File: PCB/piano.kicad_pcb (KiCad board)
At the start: 2 copper layers, 100 x 90 mm, 35 parts, among them J1 Conn_01x02, J2 Conn_01x04, J3 Conn_01x04, SW1 0, SW10 9, SW11 A, SW12 B, SW13 C, SW14 D, SW15 E, SW16 F, SW2 1, SW3 2, SW4 3, SW5 4, SW6 5, SW7 6, SW8 7, SW9 8, U1 WeMos_D1_mini

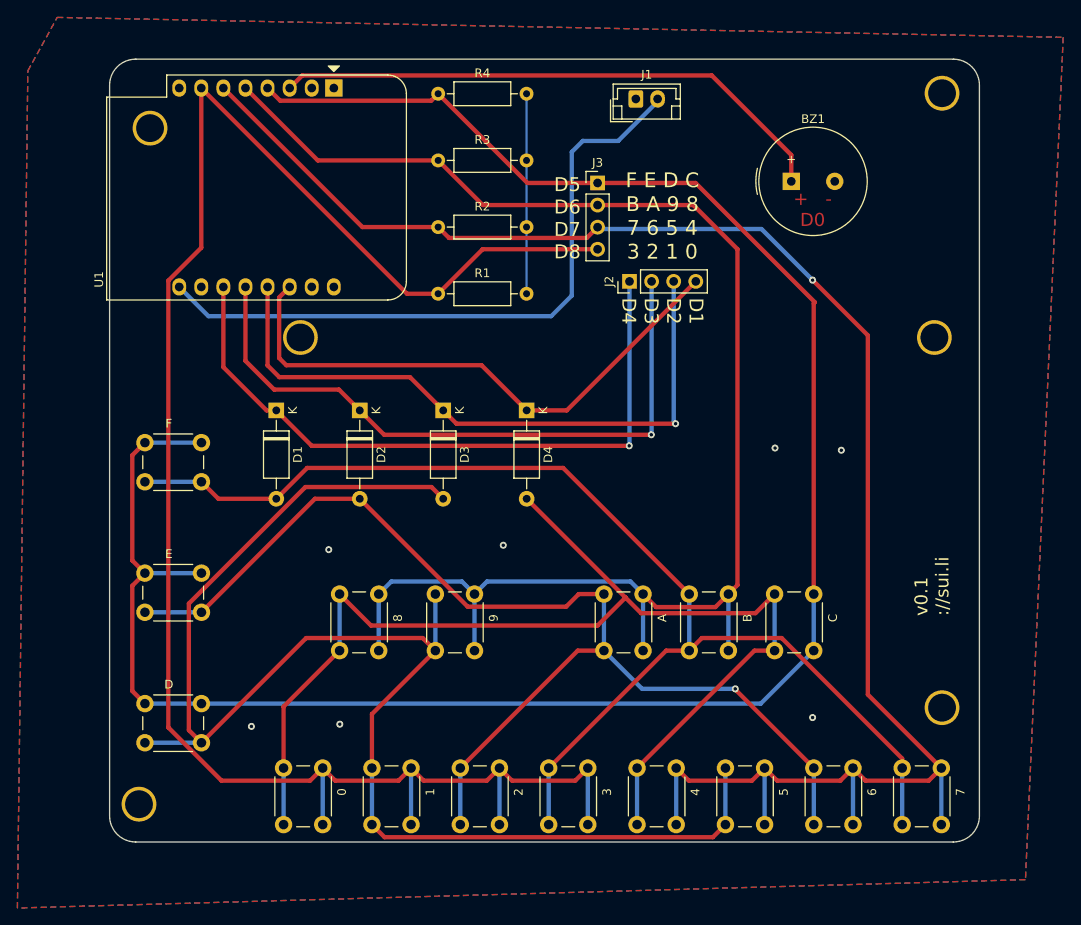
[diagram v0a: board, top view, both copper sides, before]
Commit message: v0.2 PCB
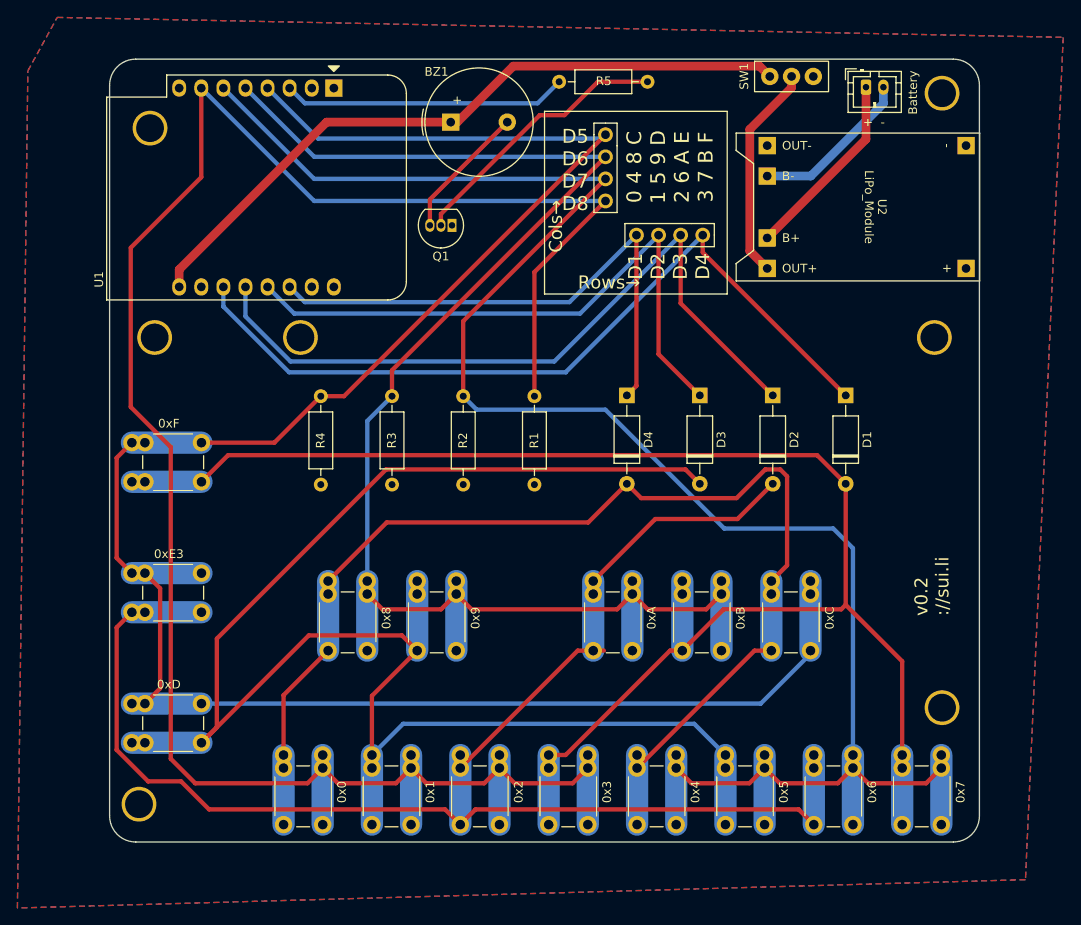
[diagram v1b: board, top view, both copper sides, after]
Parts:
- added ?: , , F.Cu at (133.7, 64.2)
- added Q1: 2N3904, Package_TO_SOT_THT:TO-92_Inline, F.Cu at (169.4, 51.1)
- added R5: 10k, Resistor_THT:R_Axial_DIN0207_L6.3mm_D2.5mm_P10.16mm_Horizontal, F.Cu at (181.7, 34.6)
- added SW1: SW_SPDT_MSM, Suat:Schiebeschalter, F.Cu at (208.4, 34.0)
- added U2: LiPo_Module, Suat:LiPoChargerModule, F.Cu at (218.3, 49.0)
- BZ1: footprint Buzzer_Beeper:Buzzer_TDK_PS1240P02BT_D12.2mm_H6.5mm -> Suat:Buzzer_D12mm_Pins6mm
- D1, D2, D3, D4: footprint Diode_THT:D_A-405_P10.16mm_Horizontal -> Suat:D_A-405_P10.16mm_Horizontal
- J1: footprint Connector_JST:JST_EH_B2B-EH-A_1x02_P2.50mm_Vertical -> Connector_JST:JST_PH_B2B-PH-K_1x02_P2.00mm_Vertical
- J2, J3: footprint Connector_PinHeader_2.54mm:PinHeader_1x04_P2.54mm_Vertical -> Suat:PinHeader_1x04_P2.54mm_Vertical_Simple
- R1, R2, R3, R4: value R -> 10k
- SW-0: renamed from SW1; value 0 -> 0x0; footprint Button_Switch_THT:SW_PUSH_6mm -> Suat:SW_PUSH_6mm
- SW-1: renamed from SW2; value 1 -> 0x1; footprint Button_Switch_THT:SW_PUSH_6mm -> Suat:SW_PUSH_6mm
- SW-2: renamed from SW3; value 2 -> 0x2; footprint Button_Switch_THT:SW_PUSH_6mm -> Suat:SW_PUSH_6mm
- SW-3: renamed from SW4; value 3 -> 0x3; footprint Button_Switch_THT:SW_PUSH_6mm -> Suat:SW_PUSH_6mm
- SW-4: renamed from SW5; value 4 -> 0x4; footprint Button_Switch_THT:SW_PUSH_6mm -> Suat:SW_PUSH_6mm
- SW-5: renamed from SW6; value 5 -> 0x5; footprint Button_Switch_THT:SW_PUSH_6mm -> Suat:SW_PUSH_6mm
- SW-6: renamed from SW7; value 6 -> 0x6; footprint Button_Switch_THT:SW_PUSH_6mm -> Suat:SW_PUSH_6mm
- SW-7: renamed from SW8; value 7 -> 0x7; footprint Button_Switch_THT:SW_PUSH_6mm -> Suat:SW_PUSH_6mm
- SW-8: renamed from SW9; value 8 -> 0x8; footprint Button_Switch_THT:SW_PUSH_6mm -> Suat:SW_PUSH_6mm
- SW-9: renamed from SW10; value 9 -> 0x9; footprint Button_Switch_THT:SW_PUSH_6mm -> Suat:SW_PUSH_6mm
- SW-A1: renamed from SW11; value A -> 0xA; footprint Button_Switch_THT:SW_PUSH_6mm -> Suat:SW_PUSH_6mm
- SW-B1: renamed from SW12; value B -> 0xB; footprint Button_Switch_THT:SW_PUSH_6mm -> Suat:SW_PUSH_6mm
- SW-C1: renamed from SW13; value C -> 0xC; footprint Button_Switch_THT:SW_PUSH_6mm -> Suat:SW_PUSH_6mm
- SW-D1: renamed from SW14; value D -> 0xD; footprint Button_Switch_THT:SW_PUSH_6mm -> Suat:SW_PUSH_6mm
- SW-E1: renamed from SW15; value E -> 0xE3; footprint Button_Switch_THT:SW_PUSH_6mm -> Suat:SW_PUSH_6mm
- SW-F1: renamed from SW16; value F -> 0xF; footprint Button_Switch_THT:SW_PUSH_6mm -> Suat:SW_PUSH_6mm
- moved D1 65.5 mm to (214.6, 70.7)
- moved D2 47.5 mm to (206.2, 70.7)
- moved BZ1 39.0 mm to (170.0, 39.2)
- moved R4 37.3 mm to (154.3, 70.8), turned to -90 degrees
- moved D3 29.5 mm to (197.9, 70.7)
- moved R3 27.6 mm to (162.5, 70.8), turned to -90 degrees
- moved J1 26.5 mm to (217.0, 35.2)
- moved R2 19.7 mm to (170.7, 70.8), turned to -90 degrees
- moved R1 16.2 mm to (178.8, 70.8), turned to -90 degrees
- moved D4 11.6 mm to (189.5, 70.7)
- moved J2 9.96 mm to (198.2, 52.2), turned to -90 degrees
- moved J3 5.62 mm to (187.0, 40.7)
- moved SW-9 2.09 mm to (165.4, 100.0)
- moved SW-8 1.32 mm to (155.1, 100.0)
- moved SW-A1 1.23 mm to (185.6, 100.0)
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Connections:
- ? pad 1: (no net) -> GND (x4)
- BZ1 pad 1: Net-(BZ1-Pad1) -> Net-(SW1-Pad1)
- BZ1 pad 2: GND -> Net-(BZ1-Pad2)
- J1 pad 1: GND -> Net-(J1-Pad1)
- REF** pad 1: (no net) -> GND (x2)
- U1 pad 3: Net-(BZ1-Pad1) -> Net-(U1-Pad3)
- U1 pad 9: Net-(J1-Pad2) -> Net-(SW1-Pad1)
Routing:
- net Net-(SW1-Pad1): track 0.00 -> 80.1 mm
- net Net-(BZ1-Pad1): track 65.1 -> 0.00 mm
- net Net-(J1-Pad2): track 76.6 -> 18.7 mm
- net Net-(D2-Pad2): track 135.3 -> 181.1 mm, vias 1 -> 0
- net Net-(D1-Pad2): track 144.0 -> 183.9 mm
- net Net-(U1-Pad3): track 0.00 -> 32.7 mm
- net D8: track 213.5 -> 246.2 mm
- net Net-(Q1-Pad2): track 0.00 -> 31.4 mm
- net Net-(D3-Pad2): track 168.8 -> 197.4 mm
- net Net-(SW1-Pad2): track 0.00 -> 24.9 mm
- net GND: track 23.0 -> 0.00 mm, vias 7 -> 0
- net D7: track 200.3 -> 222.7 mm, vias 1 -> 0
- net Net-(J1-Pad1): track 0.00 -> 22.0 mm
- net Net-(BZ1-Pad2): track 0.00 -> 15.6 mm
- net D4: track 78.5 -> 92.3 mm, vias 1 -> 0
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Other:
- board text added: "+ -"
- board text added: "0 4 8 C 1 5 9 D 2 6 A E 3 7 B F"
- board text added: "Cols→"
- board text added: "Rows→"
- board text added: "v0.2 ://sui.li"
- board text removed: "+ - D0"
- board text removed: "F E D C B A 9 8 7 6 5 4 3 2 1 0"
- board text removed: "v0.1 ://sui.li"
